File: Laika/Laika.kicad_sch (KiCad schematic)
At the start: 29 parts, among them J1 A-DF_09_A_KG-T4S, J2 Micro_SD_Card, J3 0436500300, U1 LSM6DSL, U2 MS5611-01BA, U3 RASPBERRY_PI_ZERO_2_W, U4 MMC5983MA, U5 H3LIS331DLTR, U6 THVD1451D

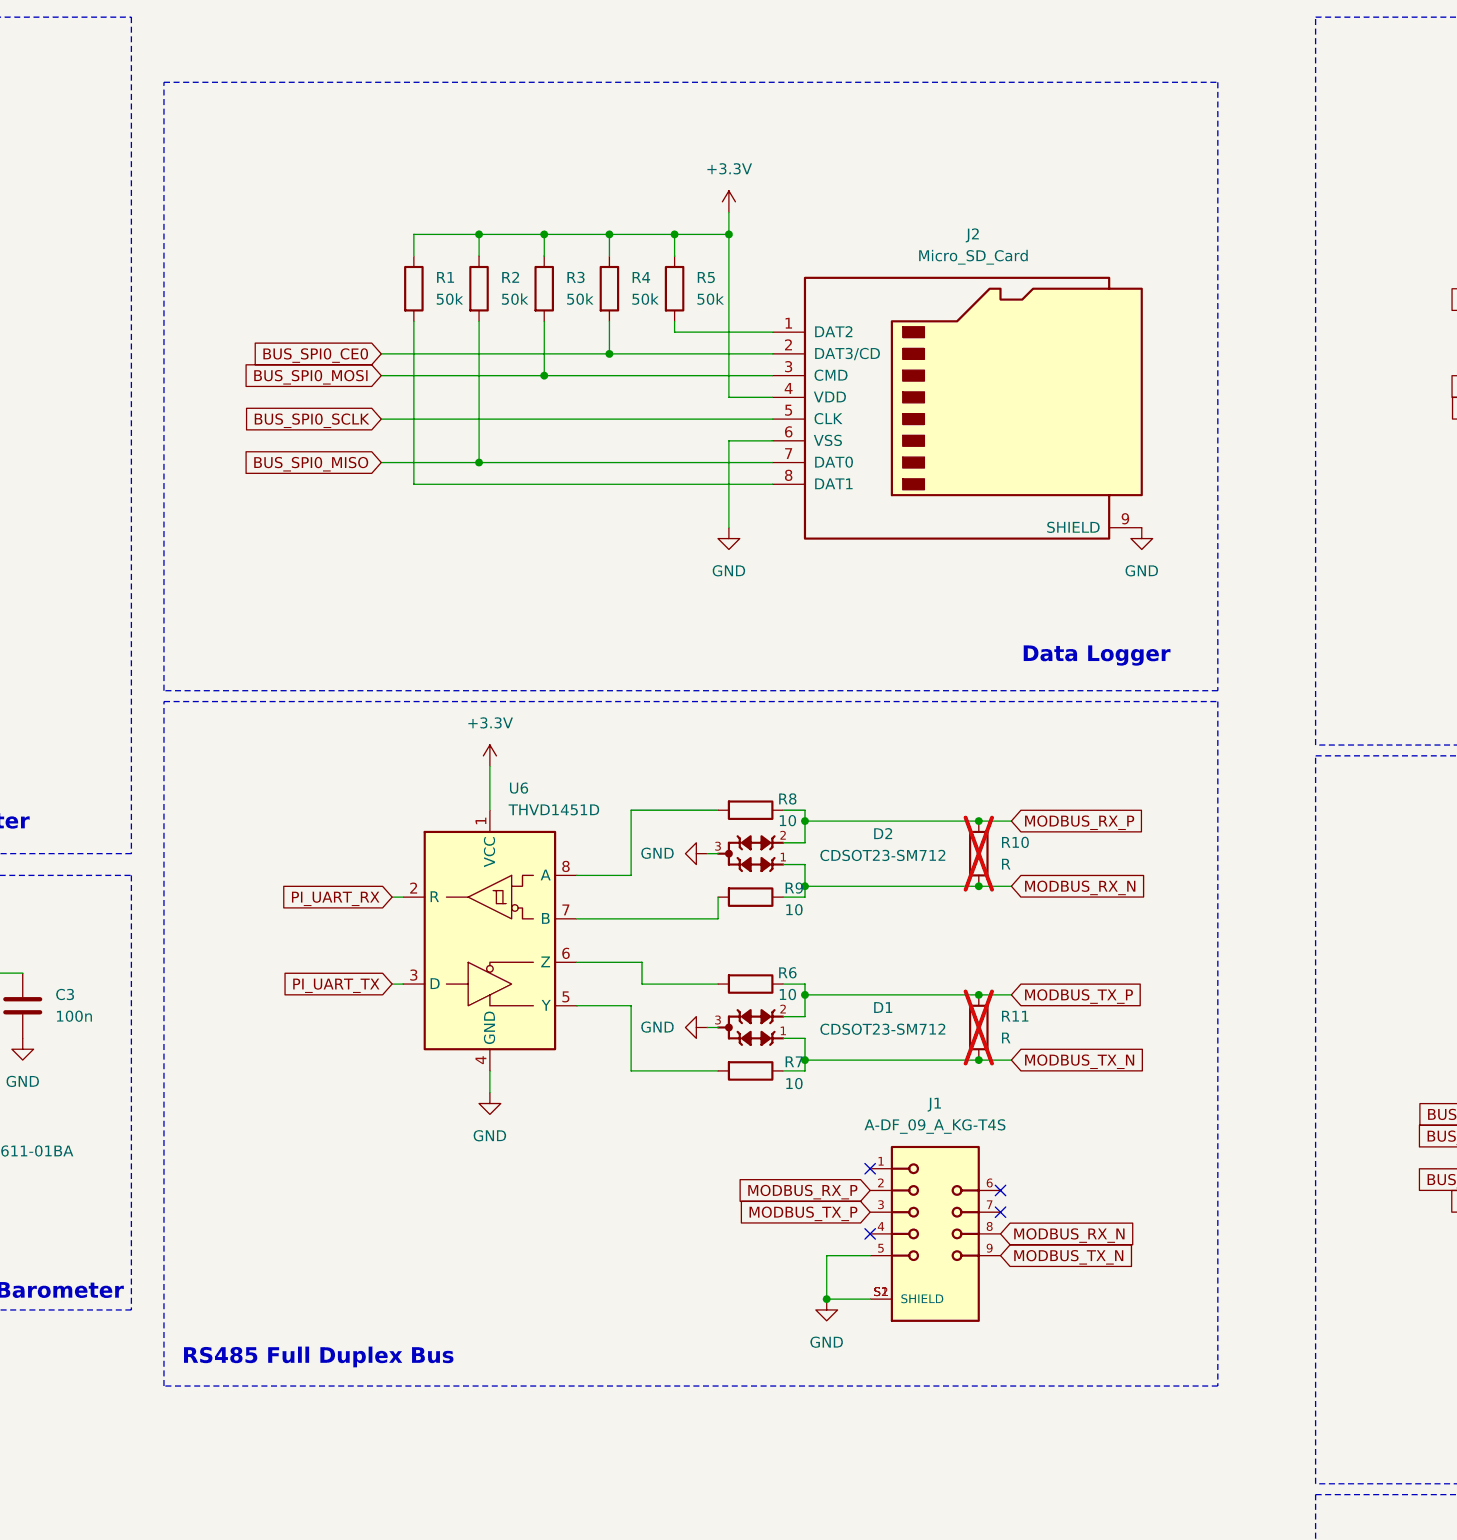
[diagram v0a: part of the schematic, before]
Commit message: Version 0A
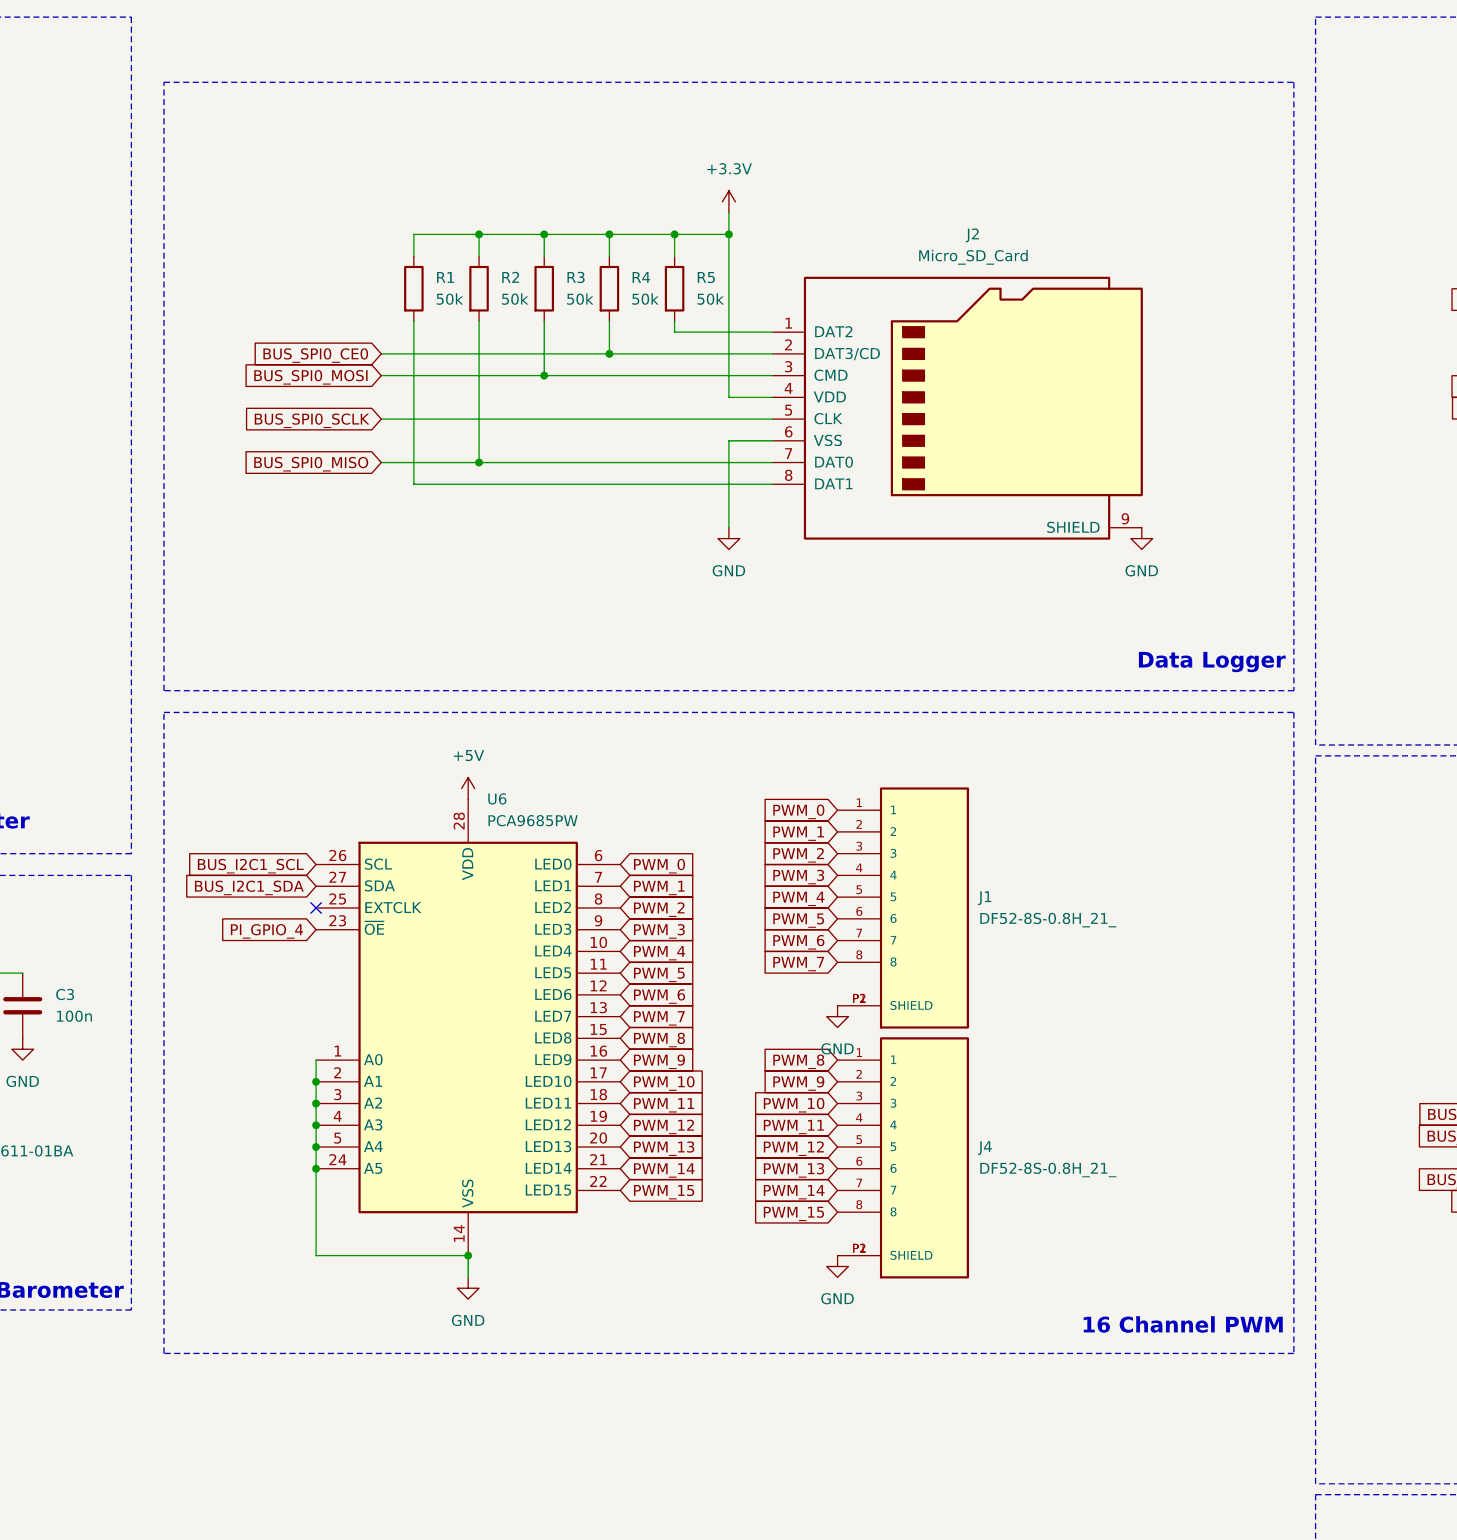
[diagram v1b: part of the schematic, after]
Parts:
- removed D1, D2: CDSOT23-SM712, CDSOT23-SM712:SOT23-3, symbol CDSOT23-SM712:CDSOT23-SM712
- removed J1: A-DF_09_A_KG-T4S, A-DF 09 AKG-T4S:ASSMANN_A-DF_09_A_KG-T4S, symbol A-DF_09_A_KG-T4S:A-DF_09_A_KG-T4S
- removed R10, R11: R, Resistor_SMD:R_1206_3216Metric, symbol Device:R
- removed R6, R7, R8, R9: 10, Resistor_SMD:R_1206_3216Metric, symbol Device:R
- removed U6: THVD1451D, Package_SO:SOIC-8_3.9x4.9mm_P1.27mm, symbol Interface_UART:THVD1451D
- added J1, J4: DF52-8S-0.8H_21_, Hirose D52:HIROSE_DF52-8S-0.8H_21_, symbol DF52-8S-0.8H_21_:DF52-8S-0.8H_21_
- added U6: PCA9685PW, Package_SO:TSSOP-28_4.4x9.7mm_P0.65mm, symbol Driver_LED:PCA9685PW
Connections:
- net +5V: now also U6.28 (VDD)
- net BUS_I2C1_SCL: now also U6.26 (SCL)
- net BUS_I2C1_SDA: now also U6.27 (SDA)
- net GND: now also J1.P1 (SHIELD), J1.P2 (SHIELD), J4.P1 (SHIELD), J4.P2 (SHIELD), U6.1 (A0), U6.14 (VSS), U6.2 (A1), U6.24 (A5), U6.3 (A2), U6.4 (A3), U6.5 (A4)
- net PI_GPIO_4: now also U6.23 (~{OE})
- new net PWM_0: J1.1, U6.6 (LED0)
- new net PWM_1: J1.2, U6.7 (LED1)
- new net PWM_10: J4.3, U6.17 (LED10)
- new net PWM_11: J4.4, U6.18 (LED11)
- new net PWM_12: J4.5, U6.19 (LED12)
- new net PWM_13: J4.6, U6.20 (LED13)
- new net PWM_14: J4.7, U6.21 (LED14)
- new net PWM_15: J4.8, U6.22 (LED15)
- new net PWM_2: J1.3, U6.8 (LED2)
- new net PWM_3: J1.4, U6.9 (LED3)
- new net PWM_4: J1.5, U6.10 (LED4)
- new net PWM_5: J1.6, U6.11 (LED5)
- new net PWM_6: J1.7, U6.12 (LED6)
- new net PWM_7: J1.8, U6.13 (LED7)
- new net PWM_8: J4.1, U6.15 (LED8)
- new net PWM_9: J4.2, U6.16 (LED9)
- no-connect marks 10 -> 7
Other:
- note added: "16 Channel PWM"
- note removed: "RS485 Full Duplex Bus"
